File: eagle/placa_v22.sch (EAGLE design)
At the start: 32 parts, among them IC1 7805, Q1 IRF740, Y1 16MHz

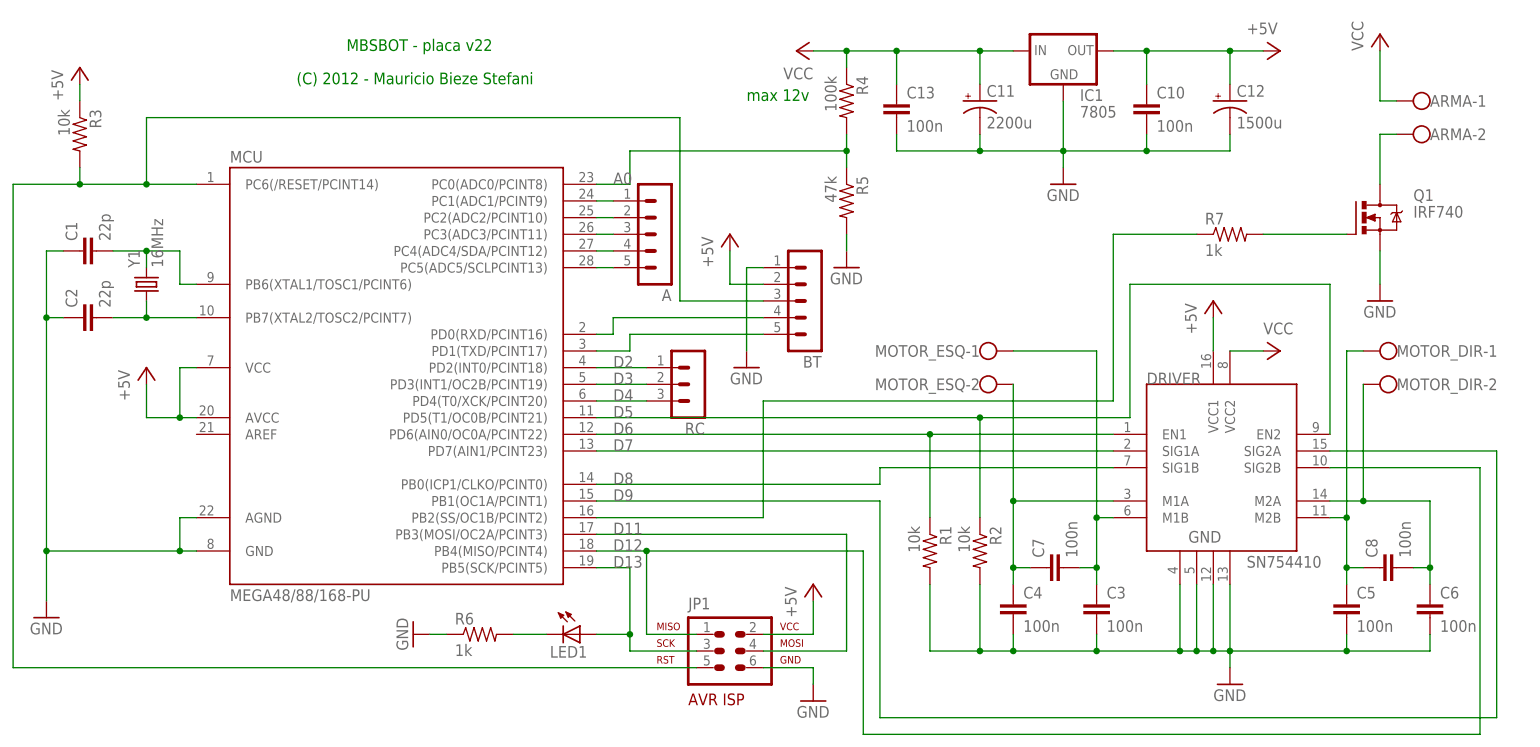
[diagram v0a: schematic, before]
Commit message: Eletronica
git-svn-id: https://mbs-bot.googlecode.com/svn/trunk@214 3c29fe3e-da84-11de-ae71-c59d11f48c9c
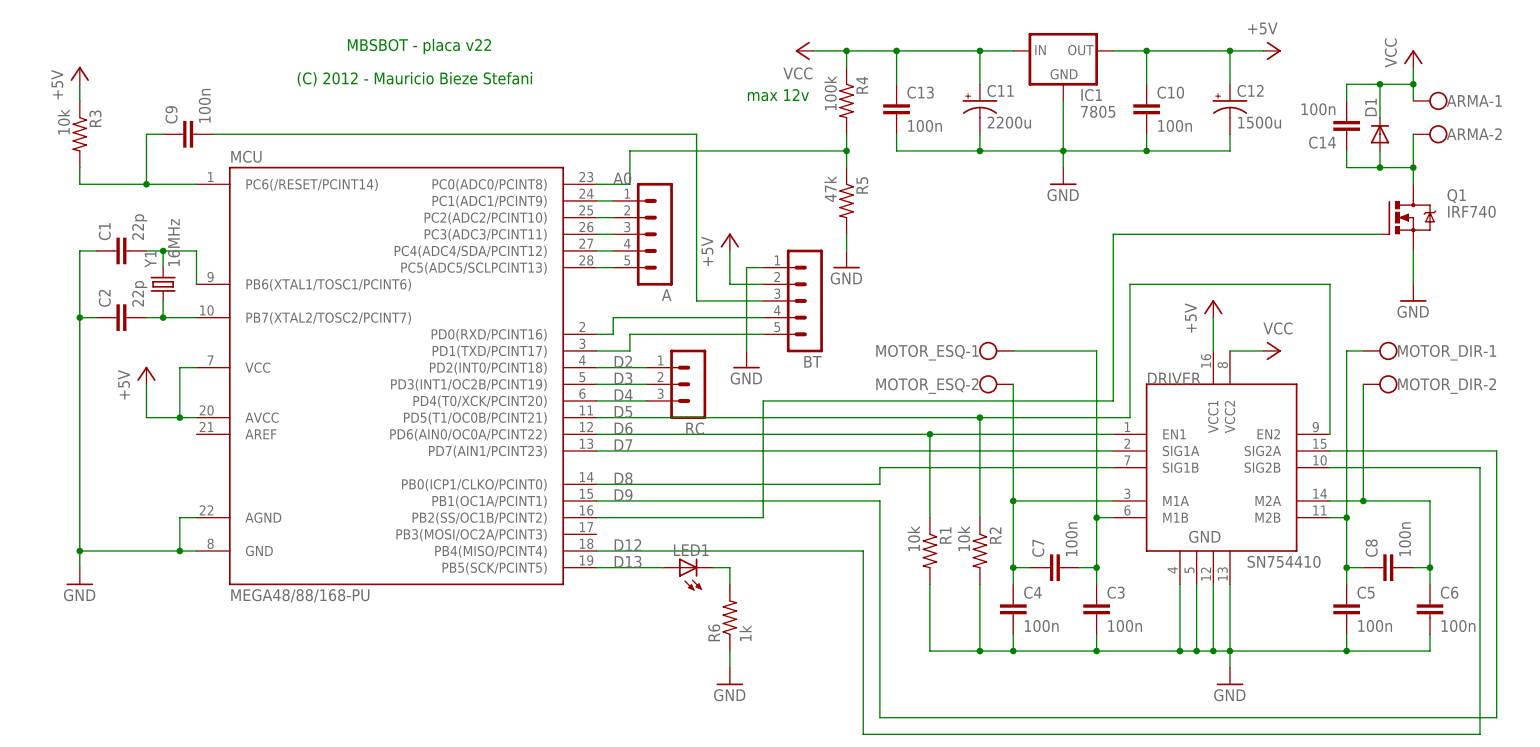
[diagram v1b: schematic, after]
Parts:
- removed JP1: AVR-ISP-6VERT, avr-7:AVR-ISP-6VERT
- removed R7: 1k, SparkFun:RESISTORKIT
- added C14, C9: 100n, SparkFun:CAPPTH1
- added D1: (no value), SparkFun:DIODEPTH
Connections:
- removed net D11: JP1.4, MCU.PB3(MOSI/OC2A/PCINT3)
- net +5V: no longer JP1.2
- net D12: no longer JP1.1
- net D13: no longer JP1.3
- net D9: now also Q1.G; no longer R7.1
- net GND: no longer JP1.6
- net N$10: now also C9.2; no longer JP1.5, MCU.PC6(/RESET/PCINT14), R3.2
- net N$11: now also C14.1, D1.A
- net N$2: now also C9.1, MCU.PC6(/RESET/PCINT14), R3.2; no longer Q1.G, R7.2
- net VCC: now also C14.2, D1.C
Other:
- moved on the sheet: ARMA-1, ARMA-2, C1, C2, LED1, Q1, R6, Y1
